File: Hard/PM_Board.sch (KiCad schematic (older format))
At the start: 63 parts, among them J1 Micro_SD_Card_Det_Hirose_DM3AT, J101 LiPo_V+, J102 LiPo_V-, J2 KRC_Conn_SWD, J3 USB_B_Micro, J4 KRC_Conn_CAN, J5 KRC_Conn_CAN, J6 KRC_Conn_CAN, Q1 SSM6J501NU, Q2 2n7002, U1 CY8C58xxLTI-LPxxx, U2 INA226, U3 NCV7342, Y1 24MHz

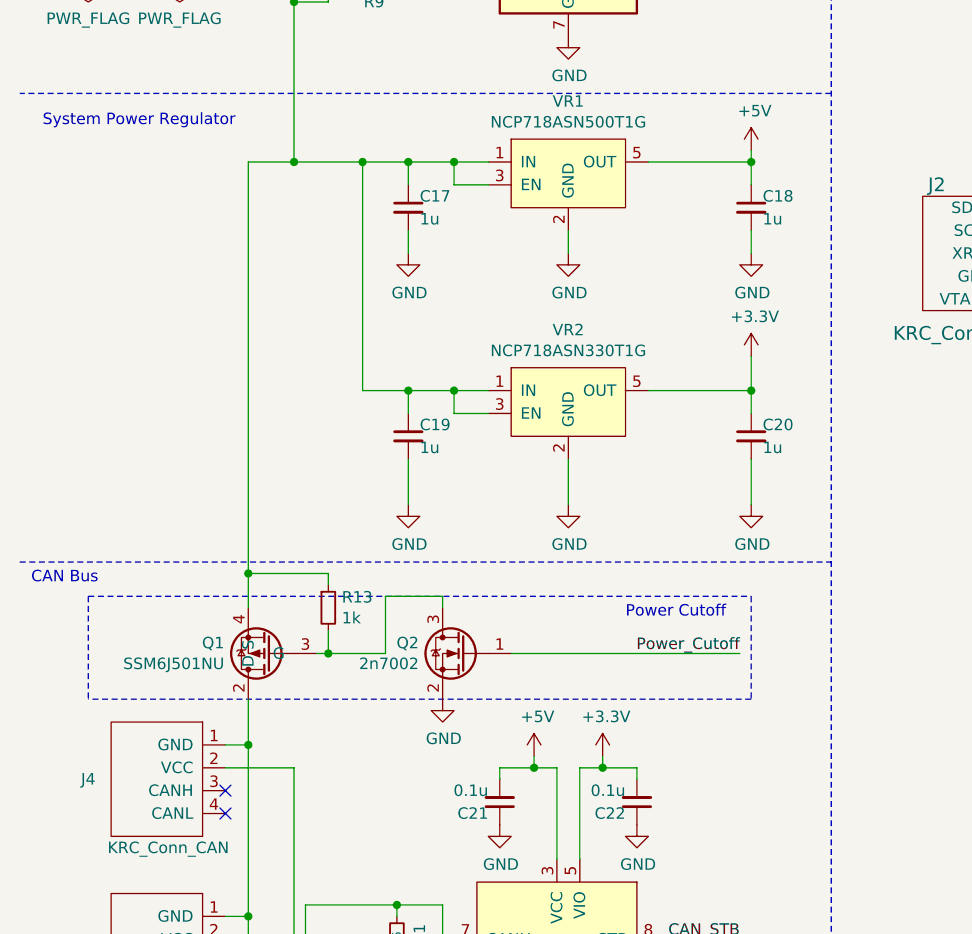
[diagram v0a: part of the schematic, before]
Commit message: [update] ミスを修正
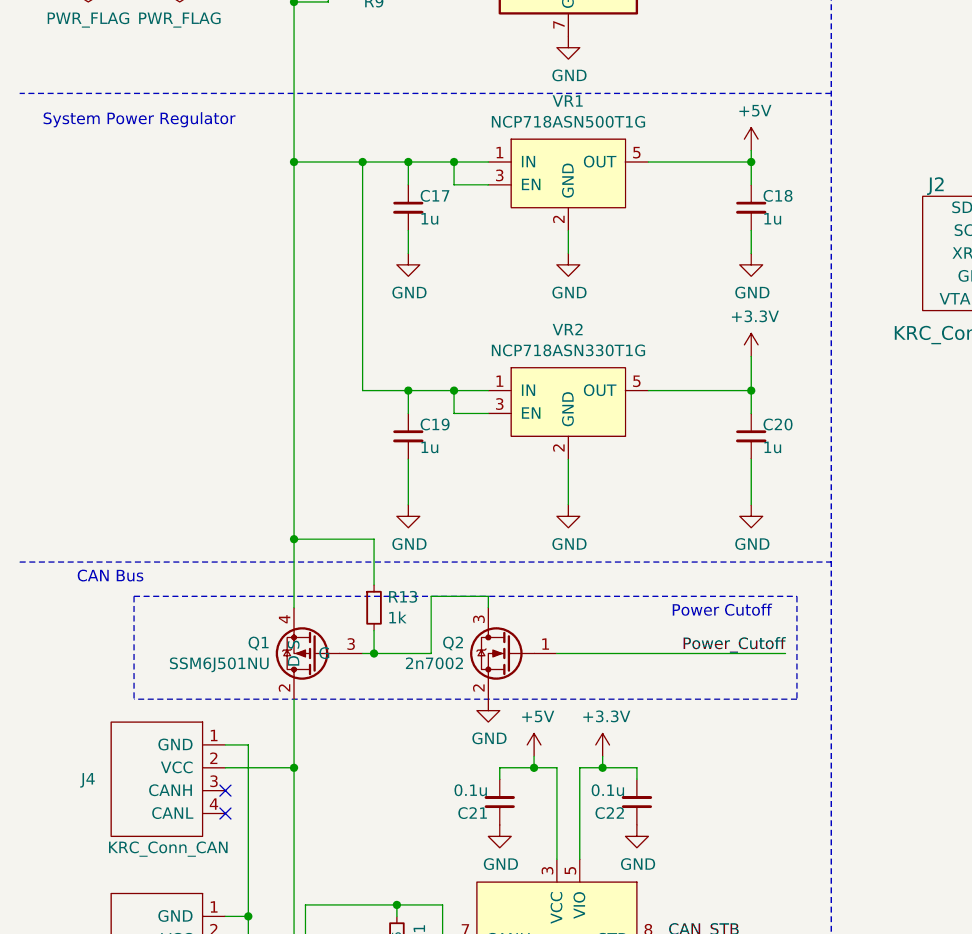
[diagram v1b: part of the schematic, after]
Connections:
- net GND: no longer Q1.1, Q1.2 (D), Q1.5, Q1.6, Q1.7
- net at J4.2 (VCC), J5.2 (VCC): now also Q1.1, Q1.2 (D), Q1.5, Q1.6, Q1.7
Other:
- moved on the sheet: Q1, Q2, R13
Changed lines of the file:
@@
 Wire Wire Line
 	1400 6050 1500 6050
-Text Label 3650 5650 2    50   ~ 0
+Text Label 3850 5650 2    50   ~ 0
 Power_Cutoff
 Text Label 3650 6900 2    50   ~ 0
@@
 Text Notes 600  3350 0    50   ~ 0
 System Power Regulator
-Text Notes 550  5350 0    50   ~ 0
+Text Notes 750  5350 0    50   ~ 0
 CAN Bus
-Text Notes 3150 5500 0    50   ~ 0
+Text Notes 3350 5500 0    50   ~ 0
 Power Cutoff
 Text Label 4850 5450 0    50   ~ 0
@@
 L Device:R_Small R13
 U 1 1 5DEF48DF
-P 1850 5450
-F 0 "R13" H 1909 5496 50  0000 L CNN
-F 1 "1k" H 1909 5405 50  0000 L CNN
-F 2 "Resistor_SMD:R_0402_1005Metric" H 1850 5450 50  0001 C CNN
-F 3 "https://b2b-api.panasonic.eu/file_stream/pids/fileversion/1242" H 1850 5450 50  0001 C CNN
-F 4 "Digikey" H 1850 5450 50  0001 C CNN "Agency"
-F 5 "ERJ-2GEJ102X" H 1850 5450 50  0001 C CNN "MPN"
-F 6 "https://www.digikey.jp/product-detail/ja/panasonic-electronic-components/ERJ-2GEJ102X/P1.0KJCT-ND/146897" H 1850 5450 50  0001 C CNN "Link"
-F 7 "1kΩ" H 1850 5450 50  0001 C CNN "Value"
-	1    1850 5450
+P 2050 5450
+F 0 "R13" H 2109 5496 50  0000 L CNN
+F 1 "1k" H 2109 5405 50  0000 L CNN
+F 2 "Resistor_SMD:R_0402_1005Metric" H 2050 5450 50  0001 C CNN
+F 3 "https://b2b-api.panasonic.eu/file_stream/pids/fileversion/1242" H 2050 5450 50  0001 C CNN
+F 4 "Digikey" H 2050 5450 50  0001 C CNN "Agency"
+F 5 "ERJ-2GEJ102X" H 2050 5450 50  0001 C CNN "MPN"
+F 6 "https://www.digikey.jp/product-detail/ja/panasonic-electronic-components/ERJ-2GEJ102X/P1.0KJCT-ND/146897" H 2050 5450 50  0001 C CNN "Link"
+F 7 "1kΩ" H 2050 5450 50  0001 C CNN "Value"
+	1    2050 5450
 	1    0    0    -1
 $EndComp
@@
 L KUTKiCad_symbol:SSM6J501NU Q1
 U 1 1 5D9715A0
-P 1500 5650
-F 0 "Q1" H 1395 5696 50  0000 R CNN
-F 1 "SSM6J501NU" H 1395 5605 50  0000 R CNN
-F 2 "KUTKiCad_footprint:UDFN6B" H 1600 5350 50  0001 C CNN
-F 3 "https://toshiba.semicon-storage.com/jp/product/mosfet/detail.SSM6J501NU.html" H 1600 5350 50  0001 C CNN
-F 4 "Digikey" H 0   0   50  0001 C CNN "Agency"
-F 5 "https://www.digikey.jp/product-detail/ja/toshiba-semiconductor-and-storage/SSM6J501NULF/SSM6J501NULFCT-ND/3191349" H 0   0   50  0001 C CNN "Link"
-F 6 "SSM6J501NU,LF" H 0   0   50  0001 C CNN "MPN"
-	1    1500 5650
+P 1700 5650
+F 0 "Q1" H 1595 5696 50  0000 R CNN
+F 1 "SSM6J501NU" H 1595 5605 50  0000 R CNN
+F 2 "KUTKiCad_footprint:UDFN6B" H 1800 5350 50  0001 C CNN
+F 3 "https://toshiba.semicon-storage.com/jp/product/mosfet/detail.SSM6J501NU.html" H 1800 5350 50  0001 C CNN
+F 4 "Digikey" H 200 0   50  0001 C CNN "Agency"
+F 5 "https://www.digikey.jp/product-detail/ja/toshiba-semiconductor-and-storage/SSM6J501NULF/SSM6J501NULFCT-ND/3191349" H 200 0   50  0001 C CNN "Link"
+F 6 "SSM6J501NU,LF" H 200 0   50  0001 C CNN "MPN"
+	1    1700 5650
 	1    0    0    -1
 $EndComp
@@
 Connection ~ 1500 6800
 $Comp
-L power:GND #PWR?
+L power:GND #PWR0135
 U 1 1 5DA49324
 P 1500 7400
-F 0 "#PWR?" H 1500 7150 50  0001 C CNN
+F 0 "#PWR0135" H 1500 7150 50  0001 C CNN
 F 1 "GND" H 1505 7227 50  0000 C CNN
 F 2 "" H 1500 7400 50  0001 C CNN
@@
 	1    0    0    -1
 $EndComp
-Wire Wire Line
-	1500 5850 1500 6050
-Connection ~ 1500 6050
 Wire Notes Line
-	800  5400 3700 5400
+	1000 5400 3900 5400
 Wire Notes Line
-	3700 5400 3700 5850
+	3900 5400 3900 5850
 Wire Notes Line
-	3700 5850 800  5850
+	3900 5850 1000 5850
 Wire Notes Line
-	800  5400 800  5850
-Wire Wire Line
-	1800 5650 1850 5650
-Wire Wire Line
-	1500 5300 1850 5300
-Wire Wire Line
-	1850 5300 1850 5350
-Connection ~ 1500 5300
-Wire Wire Line
-	1500 5300 1500 5450
-Wire Wire Line
-	1850 5550 1850 5650
-Wire Wire Line
-	1500 3500 1500 5300
-Wire Wire Line
-	1500 3500 1700 3500
-Connection ~ 1700 3500
+	1000 5400 1000 5850
+Wire Wire Line
+	2000 5650 2050 5650
+Wire Wire Line
+	2050 5550 2050 5650
 Wire Wire Line
 	1700 3500 2000 3500
@@
 L Device:Q_NMOS_GSD Q2
 U 1 1 5DB5D4F9
-P 2450 5650
-F 0 "Q2" H 2654 5696 50  0000 L CNN
-F 1 "2n7002" H 2654 5605 50  0000 L CNN
-F 2 "Package_TO_SOT_SMD:SOT-23" H 2650 5750 50  0001 C CNN
-F 3 "http://akizukidenshi.com/download/2n7002.pdf" H 2450 5650 50  0001 C CNN
-F 4 "秋月電子" H 0   0   50  0001 C CNN "Agency"
-F 5 "http://akizukidenshi.com/catalog/g/gI-03919/" H 0   0   50  0001 C CNN "Link"
-F 6 "2N7002" H 0   0   50  0001 C CNN "MPN"
-	1    2450 5650
+P 2650 5650
+F 0 "Q2" H 2854 5696 50  0000 L CNN
+F 1 "2n7002" H 2854 5605 50  0000 L CNN
+F 2 "Package_TO_SOT_SMD:SOT-23" H 2850 5750 50  0001 C CNN
+F 3 "http://akizukidenshi.com/download/2n7002.pdf" H 2650 5650 50  0001 C CNN
+F 4 "秋月電子" H 200 0   50  0001 C CNN "Agency"
+F 5 "http://akizukidenshi.com/catalog/g/gI-03919/" H 200 0   50  0001 C CNN "Link"
+F 6 "2N7002" H 200 0   50  0001 C CNN "MPN"
+	1    2650 5650
 	-1   0    0    -1
 $EndComp
 Wire Wire Line
-	1850 5650 2100 5650
-Wire Wire Line
-	2100 5650 2100 5400
-Wire Wire Line
-	2100 5400 2350 5400
-Connection ~ 1850 5650
-Wire Wire Line
-	2350 5400 2350 5450
-$Comp
-L power:GND #PWR?
+	2050 5650 2300 5650
+Wire Wire Line
+	2300 5650 2300 5400
+Wire Wire Line
+	2300 5400 2550 5400
+Connection ~ 2050 5650
+Wire Wire Line
+	2550 5400 2550 5450
+$Comp
+L power:GND #PWR0136
 U 1 1 5DC40C83
-P 2350 5850
-F 0 "#PWR?" H 2350 5600 50  0001 C CNN
-F 1 "GND" H 2355 5677 50  0000 C CNN
-F 2 "" H 2350 5850 50  0001 C CNN
-F 3 "" H 2350 5850 50  0001 C CNN
-	1    2350 5850
-	1    0    0    -1
-$EndComp
-Wire Wire Line
-	2650 5650 3650 5650
+P 2550 5850
+F 0 "#PWR0136" H 2550 5600 50  0001 C CNN
+F 1 "GND" H 2555 5677 50  0000 C CNN
+F 2 "" H 2550 5850 50  0001 C CNN
+F 3 "" H 2550 5850 50  0001 C CNN
+	1    2550 5850
+	1    0    0    -1
+$EndComp
+Wire Wire Line
+	2850 5650 3850 5650
+Wire Wire Line
+	1700 3500 1700 5150
+Connection ~ 1700 3500
+Wire Wire Line
+	1700 5850 1700 6150
+Connection ~ 1700 6150
+Wire Wire Line
+	2050 5150 1700 5150
+Wire Wire Line
+	2050 5150 2050 5350
+Connection ~ 1700 5150
+Wire Wire Line
+	1700 5150 1700 5450
 $EndSCHEMATC
